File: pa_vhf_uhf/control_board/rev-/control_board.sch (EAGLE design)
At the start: 122 parts, among them IC1 W5500, IC2 74AHC1G125DBV, IC3 ATMEGA32U4-AU, J1 USB_B_PTH, K1 G5V1, K2 G5V1, K3 G5V1, SW1 SPST_TACT-KMR2, Y1 8MHz, Y2 25MHz

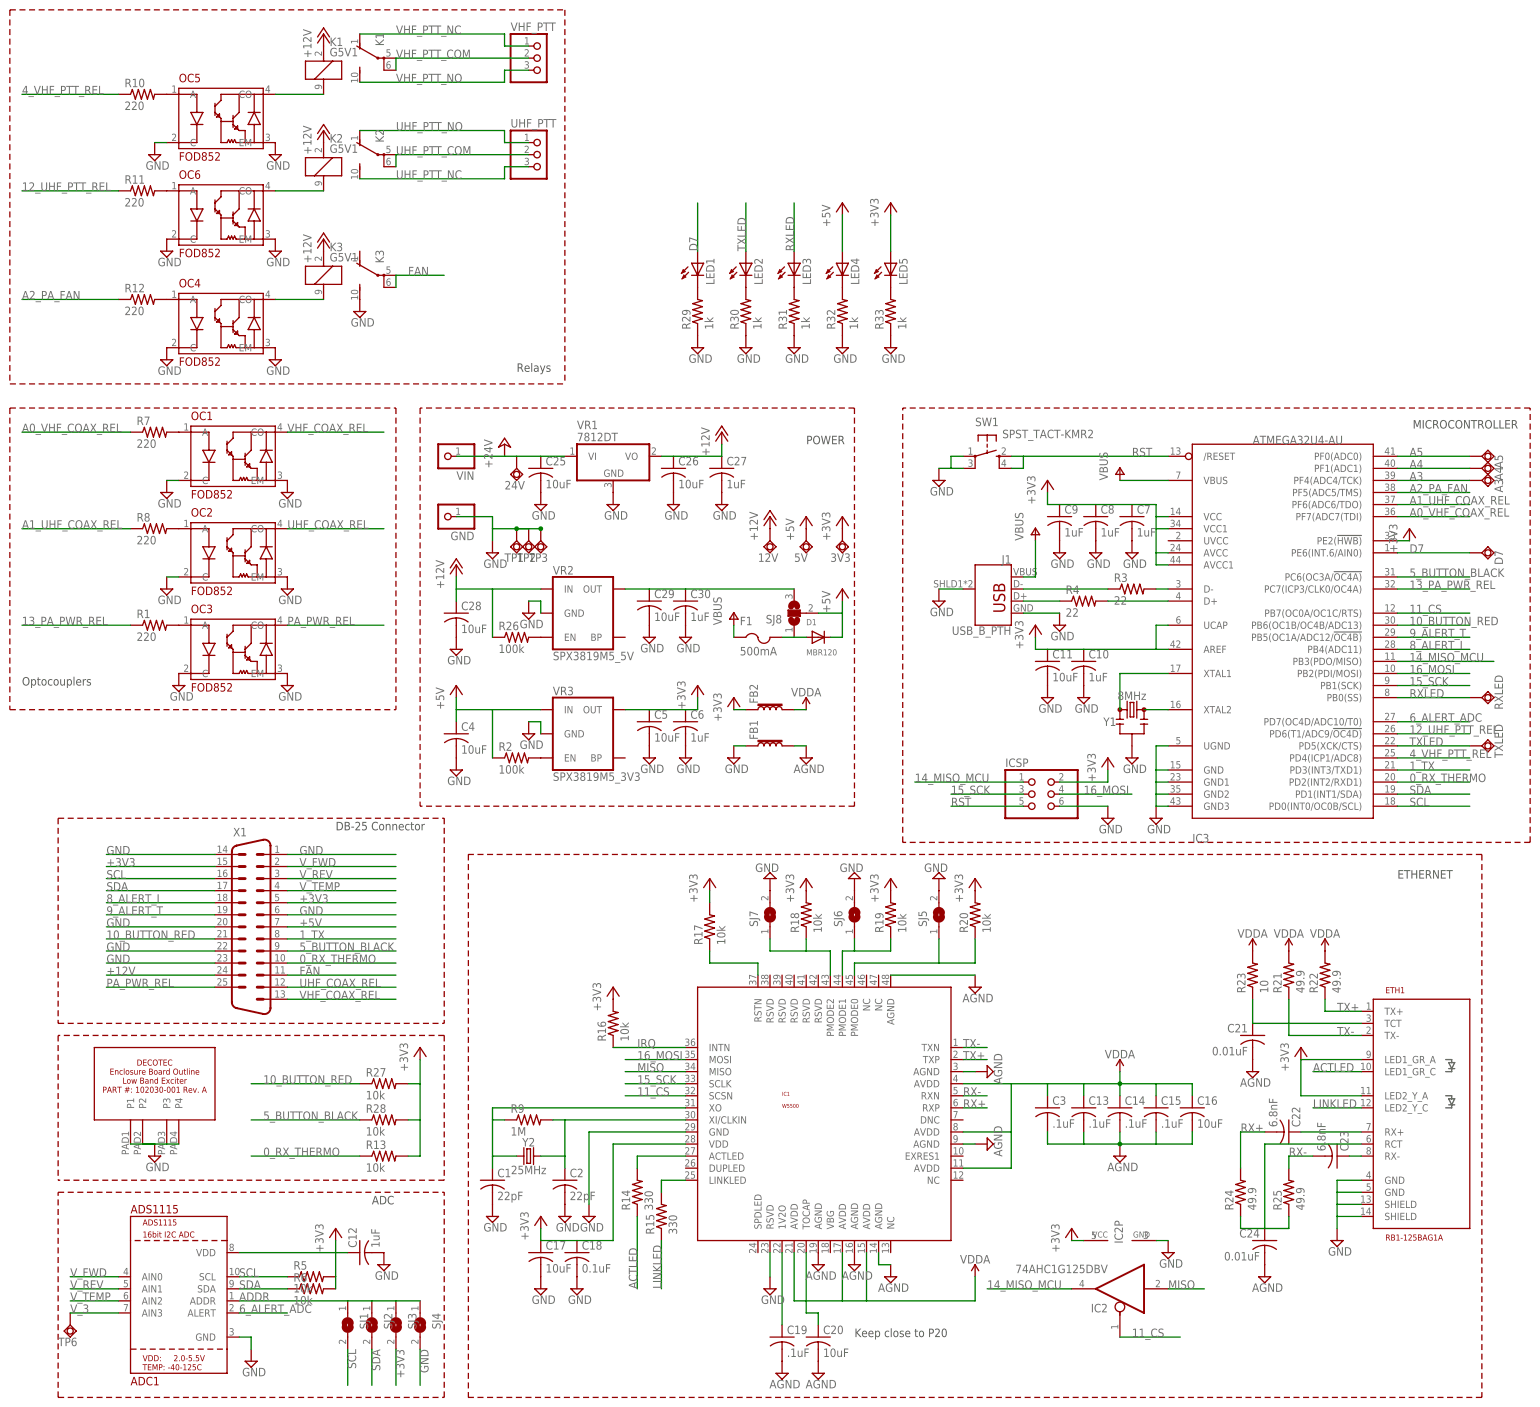
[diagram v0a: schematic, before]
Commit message: Final Commit for Rev-.  This version submitted to osh park for fab.
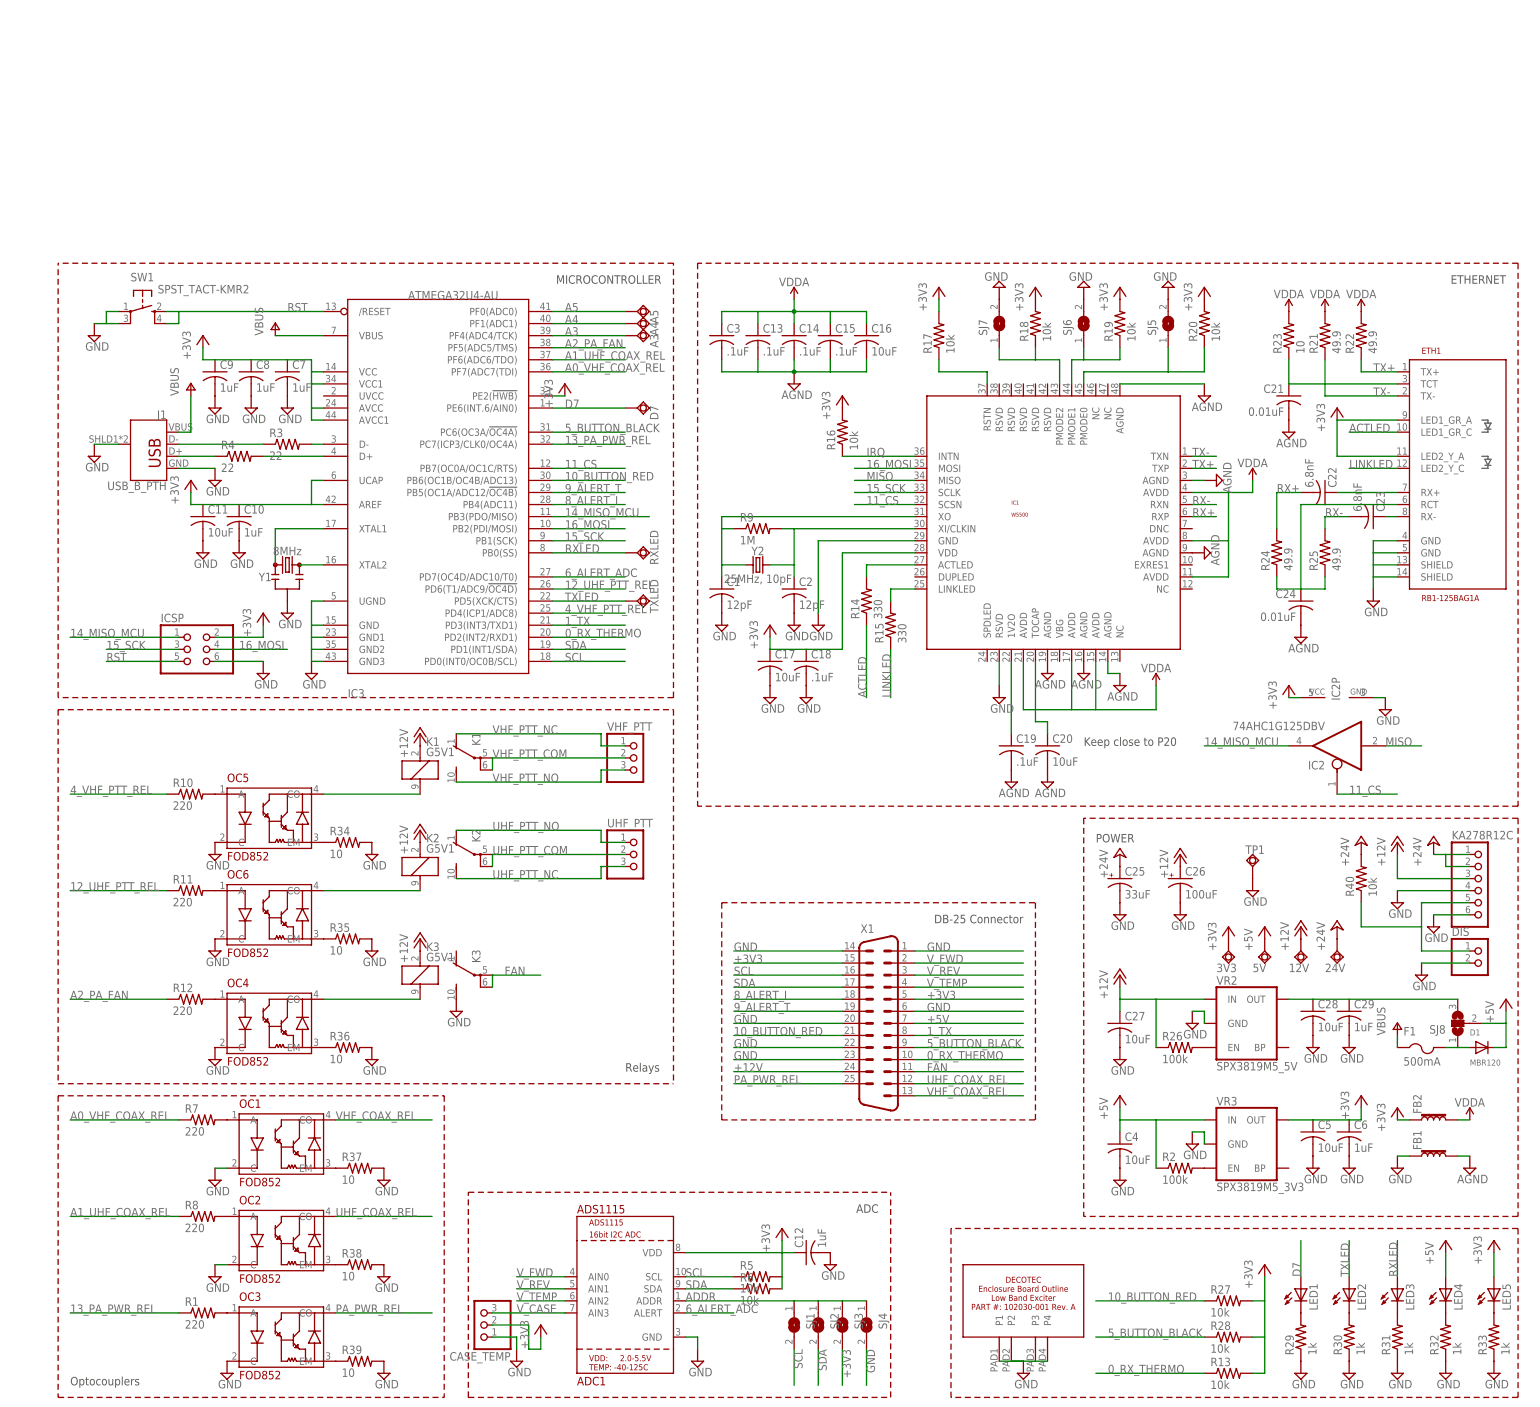
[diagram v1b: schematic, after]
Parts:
- removed C30: 1uF, rcl:C-USC0805K
- removed GND, VIN: (no value), pinhead:PINHD-1X1
- removed TP2, TP3, TP6: TPSQTP20SQ, testpad:TPSQTP20SQ
- removed VR1: 7812DT, adafruit:7812DT
- added CASE_TEMP: (no value), pinhead:PINHD-1X3
- added DIS: (no value), pinhead:PINHD-1X2
- added KA278R12C: (no value), pinhead:PINHD-1X6
- added R34, R35, R36, R37, R38, R39: 10, rcl:R-US_R0805
- added R40: 10k, rcl:R-US_R0805
- A3, A4, A5, D7, IC3, ICSP, J1, RXLED, TXLED: SPICEPREFIX (none) -> X
- C1, C2: value 22pF -> 12pF
- C18: value 0.1uF -> .1uF
- C25: value 10uF -> 33uF; device rcl:C-USC0805K -> rcl:CPOL-USC
- C26: value 10uF -> 100uF; device rcl:C-USC0805K -> rcl:CPOL-USD
- C27: value 1uF -> 10uF
- C29: value 10uF -> 1uF
- SW1: SPICEPREFIX (none) -> S
- Y1: SPICEPREFIX (none) -> J
- Y2: value 25MHz -> 25MHz, 10pF
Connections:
- removed net V_3: ADC1.AIN3, TP6.TP
- new net N$25: OC5.EM, R34.1
- new net N$26: OC6.EM, R35.1
- new net N$27: OC4.EM, R36.1
- new net N$28: OC1.EM, R37.1
- new net N$32: OC2.EM, R38.1
- new net N$40: OC3.EM, R39.1
- new net N$41: DIS.1, KA278R12C.5, R40.1
- new net V_CASE: ADC1.AIN3, CASE_TEMP.3
- net +12V: now also C26.+, KA278R12C.3; no longer C26.1, C28.1, VR1.VO
- net +24V: now also C25.+, KA278R12C.1, KA278R12C.2, R40.2; no longer C25.1, VIN.1, VR1.VI
- net +3V3: now also CASE_TEMP.2
- net GND: now also C25.-, C26.-, CASE_TEMP.1, DIS.2, KA278R12C.4, KA278R12C.6, R34.2, R35.2, R36.2, R37.2, R38.2, R39.2; no longer C25.2, C26.2, C30.2, GND.1, OC1.EM, OC2.EM, OC3.EM, OC4.EM, OC5.EM, OC6.EM, TP2.TP, TP3.TP, VR1.GND
- net N$31: now also C28.1; no longer C30.1
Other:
- moved on the sheet: 12V, 24V, 3V3, 5V, A3, A4, A5, ADC1, C1, C10, C11, C12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
